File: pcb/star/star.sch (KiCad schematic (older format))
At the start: 25 parts, among them J1 POWER, U1 ESP-12F, U2 AP2112K-3.3

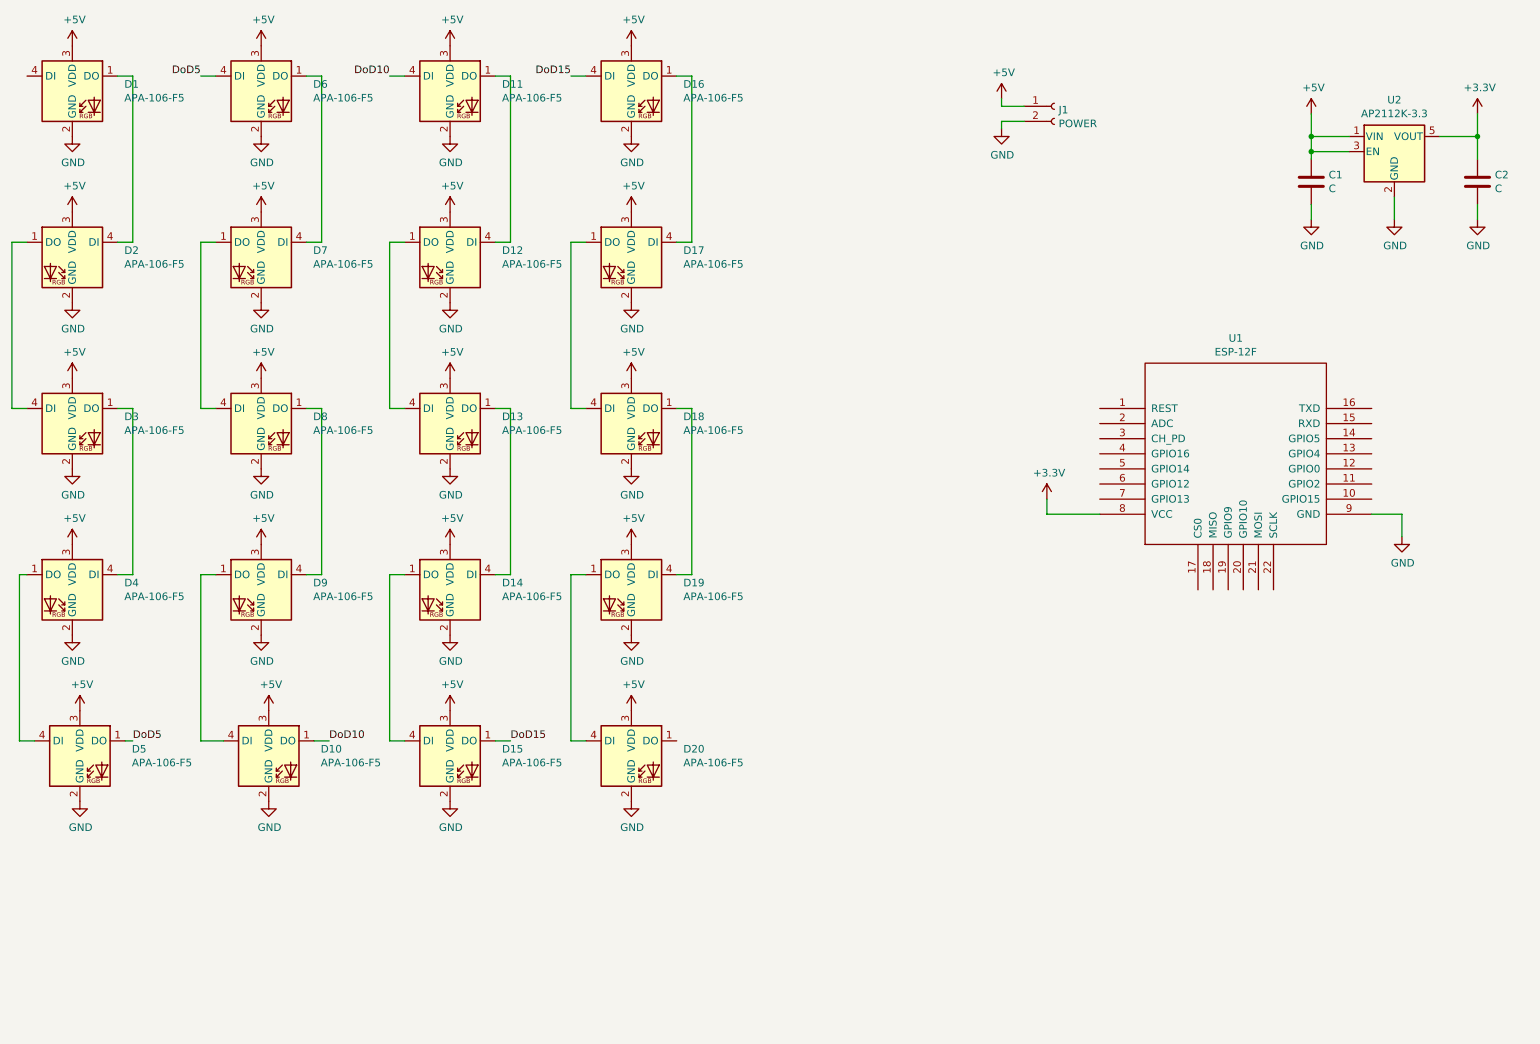
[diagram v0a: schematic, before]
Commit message: layout first pass done
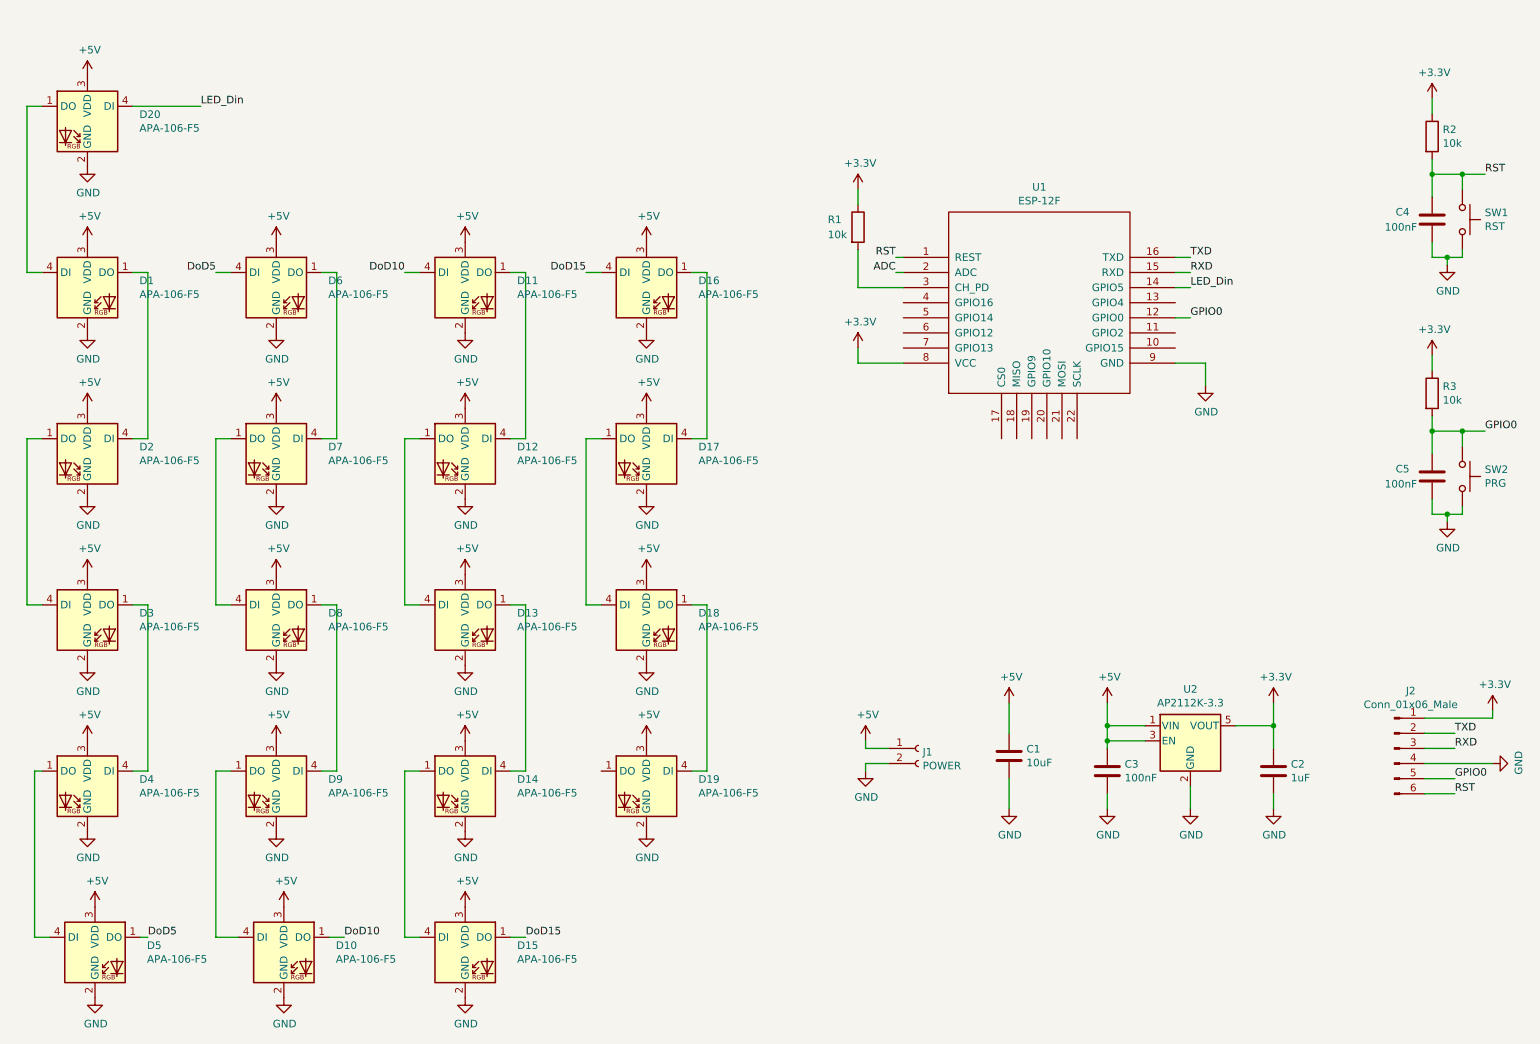
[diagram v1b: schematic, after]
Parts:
- added C3, C4, C5: 100nF, Capacitor_THT:C_Disc_D5.0mm_W2.5mm_P2.50mm, symbol Device:C
- added J2: Conn_01x06_Male, symbol Connector:Conn_01x06_Male
- added R1, R2, R3: 10k, Resistor_THT:R_Axial_DIN0204_L3.6mm_D1.6mm_P7.62mm_Horizontal, symbol Device:R
- added SW1: RST, Button_Switch_SMD:SW_SPST_EVQPE1, symbol Switch:SW_Push
- added SW2: PRG, Button_Switch_SMD:SW_SPST_EVQPE1, symbol Switch:SW_Push
- C1: value C -> 10uF; footprint (none) -> Capacitor_THT:CP_Radial_D5.0mm_P2.50mm
- C2: value C -> 1uF; footprint (none) -> Capacitor_THT:CP_Radial_D5.0mm_P2.50mm
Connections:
- net +3V3: now also J2.1 (Pin_1), R1.1, R2.1, R3.1
- net +5V: now also C3.1
- net GND: now also C3.2, C4.1, C5.1, J2.4 (Pin_4), SW1.2, SW2.2
- net RST: now reaches U1.1 (REST)
- net RST: now also C4.2, J2.6 (Pin_6), R2.2, SW1.1
- net GPIO0: now reaches U1.12 (GPIO0)
- net GPIO0: now also C5.2, J2.5 (Pin_5), R3.2, SW2.1
- net LED_Din: now reaches U1.14 (GPIO5)
- net LED_Din: now also D20.4 (DI)
- net RXD: now reaches U1.15 (RXD)
- net RXD: now also J2.3 (Pin_3)
- net TXD: now reaches U1.16 (TXD)
- net TXD: now also J2.2 (Pin_2)
- net ADC: now reaches U1.2 (ADC)
- net at U1.3 (CH_PD): now also R1.2
- net at D1.4 (DI): now also D20.1 (DO)
- net at D19.1 (DO): no longer D20.4 (DI)
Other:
- moved on the sheet: C2, D1, D10, D11, D12, D13, D14, D15, D16, D17, D18, D19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
